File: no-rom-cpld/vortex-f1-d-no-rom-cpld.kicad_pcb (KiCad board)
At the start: 2 copper layers, 80 x 50 mm, 50 parts, among them J1 JTAG, J2 CONFIG, U1 FDC 9229, U2 XC9572XL, U3 AZ1117-3.3, U4 uPD765AC, U5 74LS06N, U6 74LS06N, U7 SN74LS07N, X1 8Mhz

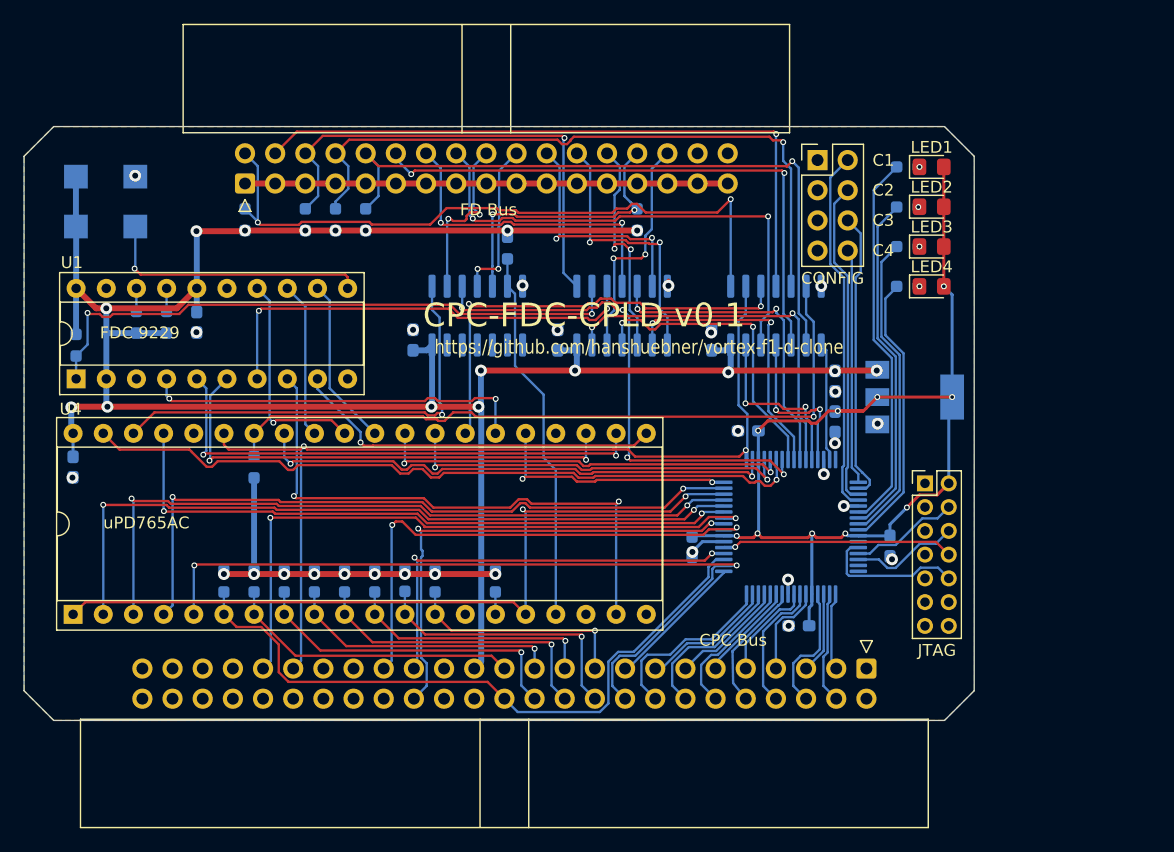
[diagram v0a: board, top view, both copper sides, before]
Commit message: cpl wip
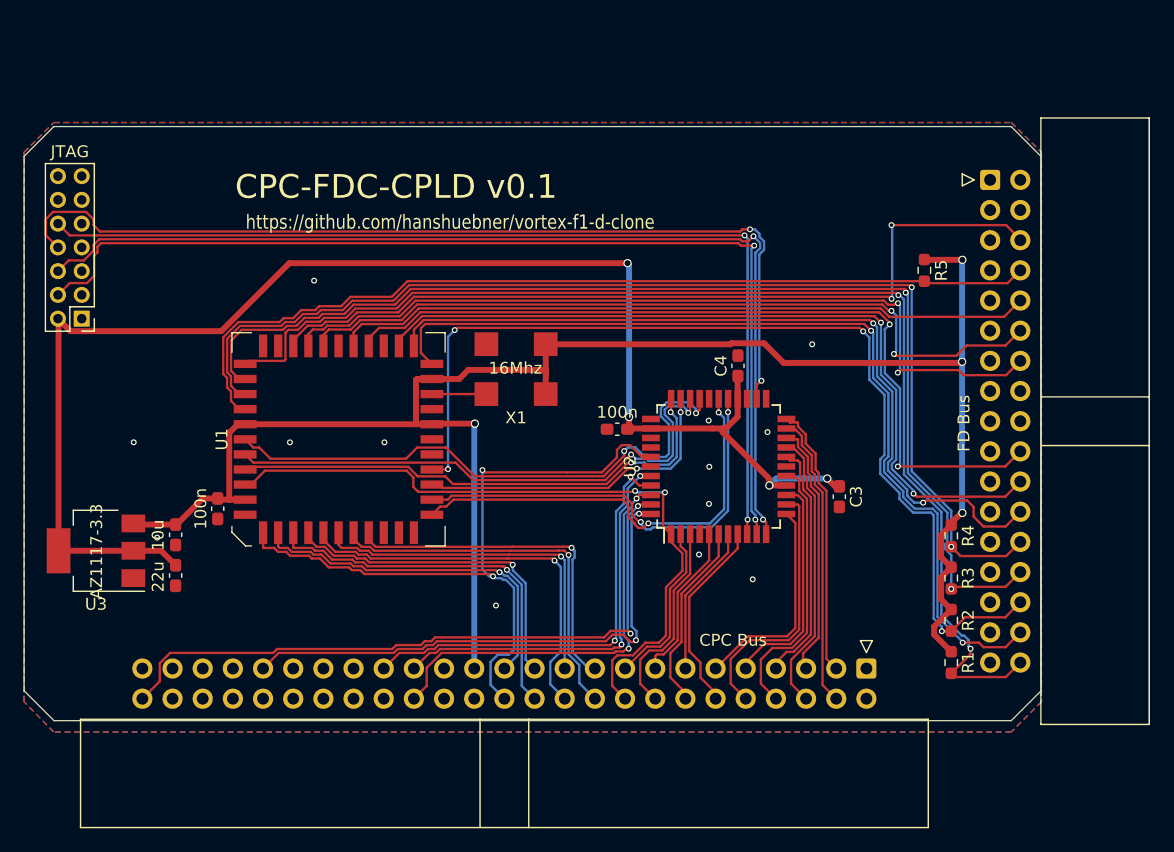
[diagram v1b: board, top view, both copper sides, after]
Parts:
- removed C5, C6, C7, C8, C9: 100n, Capacitor_SMD:C_0603_1608Metric_Pad1.08x0.95mm_HandSolder
- removed J2: CONFIG, Connector_PinHeader_2.54mm:PinHeader_2x04_P2.54mm_Vertical
- removed LED1: LED1, LED_SMD:LED_0805_2012Metric_Pad1.15x1.40mm_HandSolder
- removed LED2: LED2, LED_SMD:LED_0805_2012Metric_Pad1.15x1.40mm_HandSolder
- removed LED3: LED3, LED_SMD:LED_0805_2012Metric_Pad1.15x1.40mm_HandSolder
- removed LED4: LED4, LED_SMD:LED_0805_2012Metric_Pad1.15x1.40mm_HandSolder
- removed R10, R11, R12, R13, R14, R15, R8, R9: 10k, Resistor_SMD:R_0603_1608Metric_Pad0.98x0.95mm_HandSolder
- removed R16, R17, R18, R19, R20, R21, R22, R23: 680, Resistor_SMD:R_0603_1608Metric_Pad0.98x0.95mm_HandSolder
- removed R6, R7: 1k, Resistor_SMD:R_0603_1608Metric_Pad0.98x0.95mm_HandSolder
- removed U4: uPD765AC, Package_DIP:DIP-40_W15.24mm_Socket
- removed U5, U6: 74LS06N, Package_SO:SOIC-14_3.9x8.7mm_P1.27mm
- removed U7: SN74LS07N, Package_SO:SOIC-14_3.9x8.7mm_P1.27mm
- C1, C10, C11, C2, C3, C4, U3: moved to F.Cu
- R1, R2, R3, R4: value 180 -> 150; moved to F.Cu
- R5: value 1k -> 150; moved to F.Cu
- U1: value FDC 9229 -> 37C65; footprint Package_DIP:DIP-20_W7.62mm_Socket -> Package_LCC:PLCC-44
- U2: value XC9572XL -> XC9572XL-VQ44; footprint Package_QFP:TQFP-64_10x10mm_P0.5mm -> Package_QFP:TQFP-44_10x10mm_P0.8mm; moved to F.Cu
- X1: value 8Mhz -> 16Mhz; moved to F.Cu
- moved J1 72.3 mm to (119.9, 106.2), turned to 180 degrees
- moved U3 70.1 mm to (121.1, 125.7), turned to 180 degrees
- moved R5 66.5 mm to (190.8, 102.1)
- moved S2 62.7 mm to (196.3, 94.5), turned to 0 degrees
- moved C1 57.0 mm to (127.8, 124.4)
- moved C2 57.0 mm to (127.8, 127.8)
- moved C10 45.9 mm to (164.9, 115.5), turned to 180 degrees
- moved R1 41.9 mm to (193.1, 135.1), turned to -90 degrees
- moved X1 37.3 mm to (156.4, 110.4), turned to 180 degrees
- moved R2 35.0 mm to (193.1, 131.6), turned to -90 degrees
- moved R3 28.2 mm to (193.1, 128.0), turned to -90 degrees
- moved U1 22.7 mm to (141.5, 116.3)
- moved R4 21.3 mm to (193.1, 124.5), turned to -90 degrees
- moved C11 15.8 mm to (131.3, 122.2)
- moved C4 15.7 mm to (175.1, 110.1), turned to 90 degrees
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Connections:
- C10 pad 1: +5V -> +3.3V
- R1 pad 1: LED1 -> +5V
- R1 pad 2: Net-(LED1-Pad1) -> ~{RDY}
- R2 pad 1: LED2 -> +5V
- R2 pad 2: Net-(LED2-Pad1) -> RDATA
- R3 pad 1: LED3 -> +5V
- R3 pad 2: Net-(LED3-Pad1) -> ~{WPT}
- R4 pad 1: LED4 -> +5V
- R4 pad 2: Net-(LED4-Pad1) -> ~{TRK00}
- R5 pad 1: Net-(R5-Pad1) -> +5V
- R5 pad 2: +5V -> ~{INDEX}
- S1 pad 39: READY -> /READY
- S1 pad 50: /CLK4 -> CLK4
- S2 pad 10: ~{TRK00} -> ~{DS0}
- S2 pad 12: ~{WGATE} -> ~{DS1}
- S2 pad 14: WDATA -> ~{DS2}
- S2 pad 16: ~{STEP} -> ~{MTRON}
- S2 pad 2: ~{RDY} -> unconnected-(S2-Pin_2-Pad2)
- S2 pad 20: ~{MTRON} -> ~{STEP}
- S2 pad 22: ~{DS2} -> WDATA
- S2 pad 24: ~{DS1} -> ~{WGATE}
- S2 pad 26: ~{DS0} -> ~{TRK00}
- S2 pad 28: ~{INDEX} -> ~{WPT}
- S2 pad 30: ~{DS3} -> RDATA
- S2 pad 32: unconnected-(S2-Pad32) -> ~{SIDE1}
- S2 pad 34: unconnected-(S2-Pad34) -> ~{RDY}
- S2 pad 4: ~{SIDE1} -> unconnected-(S2-Pin_4-Pad4)
- S2 pad 6: RDATA -> ~{DS3}
- S2 pad 8: ~{WPT} -> ~{INDEX}
- U1 pad 1: RDATA' -> ~{IORD}
- U1 pad 10: GND -> /D3
- U1 pad 11: ~{CLKIN} -> /D4
- U1 pad 12: Net-(U1-Pad12) -> /D5
- U1 pad 13: Net-(U1-Pad13) -> /D6
- U1 pad 14: Net-(U1-Pad14) -> /D7
- U1 pad 16: +5V -> unconnected-(U1-IRQ-Pad16)
- U1 pad 17: Net-(R6-Pad1) -> unconnected-(U1-~{DCHGEN}-Pad17)
- U1 pad 18: Net-(R5-Pad1) -> ~{LDOR}
- U1 pad 19: GND -> ~{LDCR}
- U1 pad 2: +5V -> ~{IOWR}
- U1 pad 20: +5V -> RESET
- U1 pad 3: GND -> ~{FDCCS}
- U1 pad 4: MFM -> A0
- U1 pad 5: Net-(U1-Pad5) -> +5V
- U1 pad 6: Net-(U1-Pad6) -> GND
- U1 pad 7: WDATA' -> D0
- U1 pad 8: Net-(U1-Pad8) -> /D1
- U1 pad 9: Net-(U1-Pad9) -> /D2
- U2 pad 1: READY -> A0
- U2 pad 10: ~{DS2'} -> TMS
- U2 pad 11: ~{DS3'} -> TCK
- U2 pad 12: STEP -> /A7
- U2 pad 13: WGATE -> /A8
- U2 pad 14: GND -> /A9
- U2 pad 15: TRK00 -> +3.3V
- U2 pad 16: unconnected-(U2-Pad16) -> /A10
- U2 pad 17: CFG4 -> GND
- U2 pad 18: CFG3 -> /A11
- U2 pad 19: CFG2 -> /A12
- U2 pad 2: FLT/TRK0 -> /A1
- U2 pad 20: CFG1 -> /A13
- U2 pad 21: GND -> /A14
- U2 pad 22: LED1 -> /A15
- U2 pad 23: LED2 -> unconnected-(U2-P16-Pad23)
- U2 pad 24: LED3 -> TDO
- U2 pad 25: LED4 -> GND
- U2 pad 27: unconnected-(U2-Pad27) -> ~{LDCR}
- U2 pad 28: TDI -> ~{LDOR}
- U2 pad 29: TMS -> MTRON
- U2 pad 3: +3.3V -> /A2
- U2 pad 30: TCK -> ~{IORD}
- U2 pad 31: unconnected-(U2-Pad31) -> ~{IOWR}
- U2 pad 32: unconnected-(U2-Pad32) -> RESET
- U2 pad 33: /A15 -> ~{FDCCS}
- U2 pad 34: /A14 -> unconnected-(U2-P24/GTS2-Pad34)
- U2 pad 35: /A13 -> +3.3V
- U2 pad 36: /A12 -> unconnected-(U2-P25/GTS1-Pad36)
- U2 pad 37: +3.3V -> unconnected-(U2-P26-Pad37)
- U2 pad 38: /A11 -> D0
- U2 pad 39: /A10 -> unconnected-(U2-P28-Pad39)
- U2 pad 4: US0 -> GND
- U2 pad 40: /A9 -> ~{IORQ}
- U2 pad 41: GND -> ~{WR}
- U2 pad 42: /A8 -> ~{RD}
- U2 pad 43: /A7 -> CLK4
- U2 pad 44: /A6 -> ~{RSET}
- U2 pad 5: US1 -> /A3
- U2 pad 6: ~{RW}/SEEK -> /A4
- U2 pad 7: MTRON -> /A5
- U2 pad 8: ~{DS0'} -> /A6
- U2 pad 9: ~{DS1'} -> TDI
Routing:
- net READY: track 80.9 -> 0.00 mm, vias 2 -> 0
- net TMS: track 9.23 -> 86.4 mm, vias 0 -> 2
- net TCK: track 9.20 -> 86.1 mm, vias 0 -> 2
- net +5V: track 227.9 -> 152.2 mm, vias 26 -> 4
- net TDI: track 12.3 -> 83.5 mm, vias 0 -> 2
- net ~{RW}/SEEK: track 62.0 -> 0.00 mm, vias 1 -> 0
- net WPT: track 61.5 -> 0.00 mm, vias 1 -> 0
- net TDO: track 19.6 -> 78.7 mm, vias 1 -> 2
- net CLK4: track 0.00 -> 56.8 mm, vias 0 -> 2
- net FLTR/STEP: track 54.6 -> 0.00 mm, vias 2 -> 0
- net ~{INDEX}: track 24.7 -> 76.7 mm, vias 2 -> 0
- net RDATA': track 51.6 -> 0.00 mm, vias 2 -> 0
- net ~{DS3}: track 19.7 -> 70.1 mm
- net GND: track 50.4 -> 0.00 mm, vias 19 -> 13
- net ~{DS2}: track 20.1 -> 69.2 mm
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- added copper zone on B.Cu, net GND
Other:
- board size 80 x 50 mm -> 85.6 x 50 mm
- board text removed: "8x10k"
- board text removed: "C1"
- board text removed: "C2"
- board text removed: "C3"
- board text removed: "C4"
